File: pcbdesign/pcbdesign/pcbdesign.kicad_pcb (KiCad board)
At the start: 2 copper layers, 50 x 50 mm, 32 parts, among them J1 Conn_01x06_Male, J2 USB_B_Micro, J3 Conn_Coaxial, SW1 SW_Push, SW2 SW_Push, U1 CMWX1ZZABZ-078, U2 LM1117ADJ

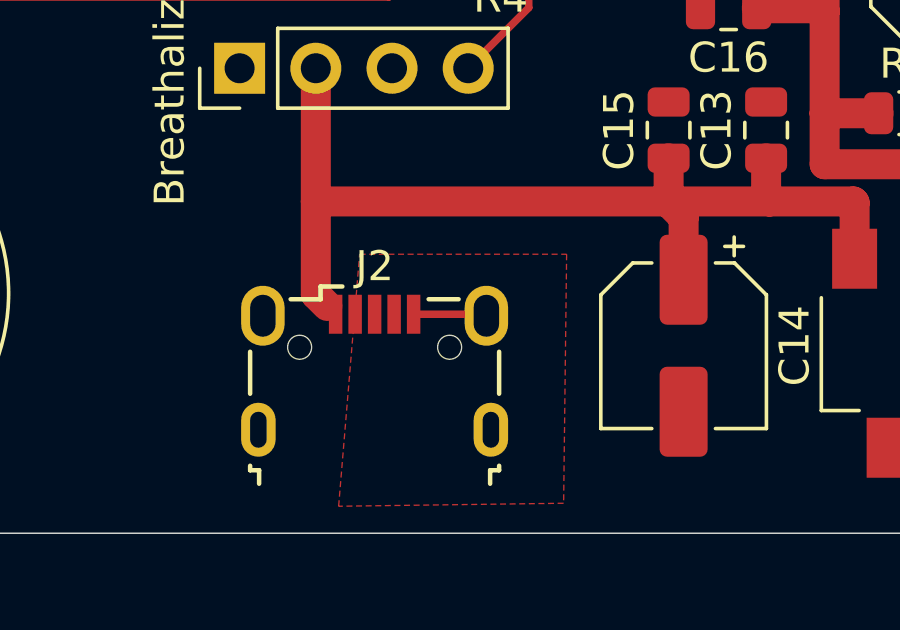
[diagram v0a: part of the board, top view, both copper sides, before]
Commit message: Update pcbdesign
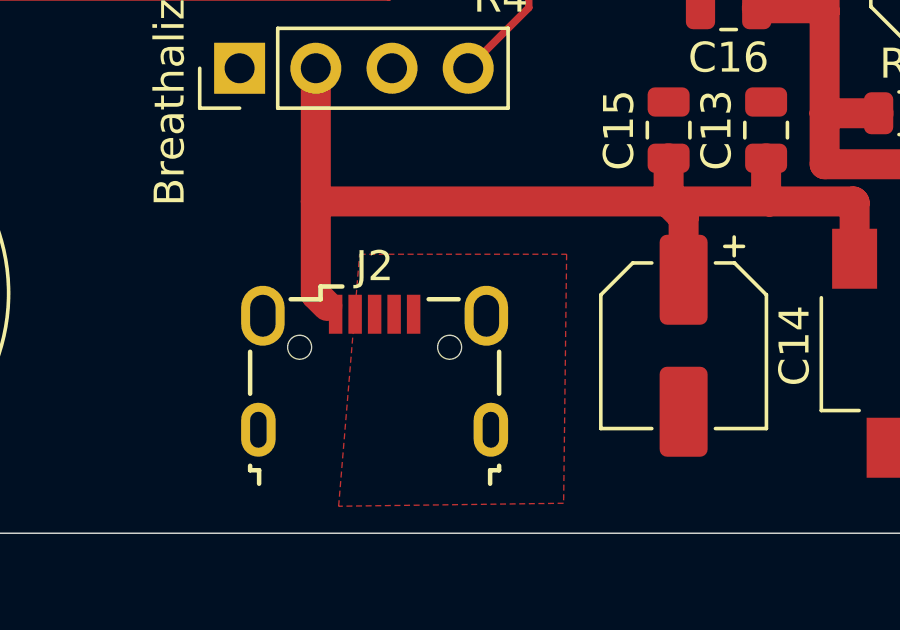
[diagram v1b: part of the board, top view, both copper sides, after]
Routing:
- net GND: track 38.8 -> 36.3 mm
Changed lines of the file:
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@@
-(kicad_pcb (version 20171130) (host pcbnew 5.1.5-1.fc31)
+(kicad_pcb (version 20171130) (host pcbnew "(5.1.5-0-10_14)")
   (general
     (thickness 1.6)
     (drawings 7)
-    (tracks 222)
+    (tracks 220)
     (zones 0)
     (modules 32)
@@
     (34 B.Paste user hide)
     (35 F.Paste user hide)
-    (36 B.SilkS user)
-    (37 F.SilkS user hide)
+    (36 B.SilkS user hide)
+    (37 F.SilkS user)
     (38 B.Mask user)
     (39 F.Mask user)
@@
     (solder_mask_min_width 0.25)
     (aux_axis_origin 0 0)
-    (visible_elements FFFFFF7F)
+    (visible_elements FFFFF77F)
     (pcbplotparams
       (layerselection 0x010d0_ffffffff)
@@
   (via (at 187.7 100.6) (size 0.8) (drill 0.4) (layers F.Cu B.Cu) (net 1))
   (segment (start 164.25 92.4) (end 164.25 93.35) (width 0.25) (layer F.Cu) (net 1))
-  (segment (start 170.375 122.7) (end 170.425 122.75) (width 0.25) (layer F.Cu) (net 1))
-  (segment (start 168 122.7) (end 170.375 122.7) (width 0.25) (layer F.Cu) (net 1))
   (segment (start 164.74 118.94) (end 176.46 118.94) (width 1) (layer F.Cu) (net 2))
   (segment (start 164.74 114.5) (end 164.74 118.94) (width 1) (layer F.Cu) (net 2))
